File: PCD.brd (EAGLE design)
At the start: 64 x 56 mm, 15 parts, among them J1 M40-SOCKET-BELOW, J2 DC IN, J4 DC IN, J5 OLED, J7 M14PTH, J8 M06-PLAIN, J9 M06-PLAIN

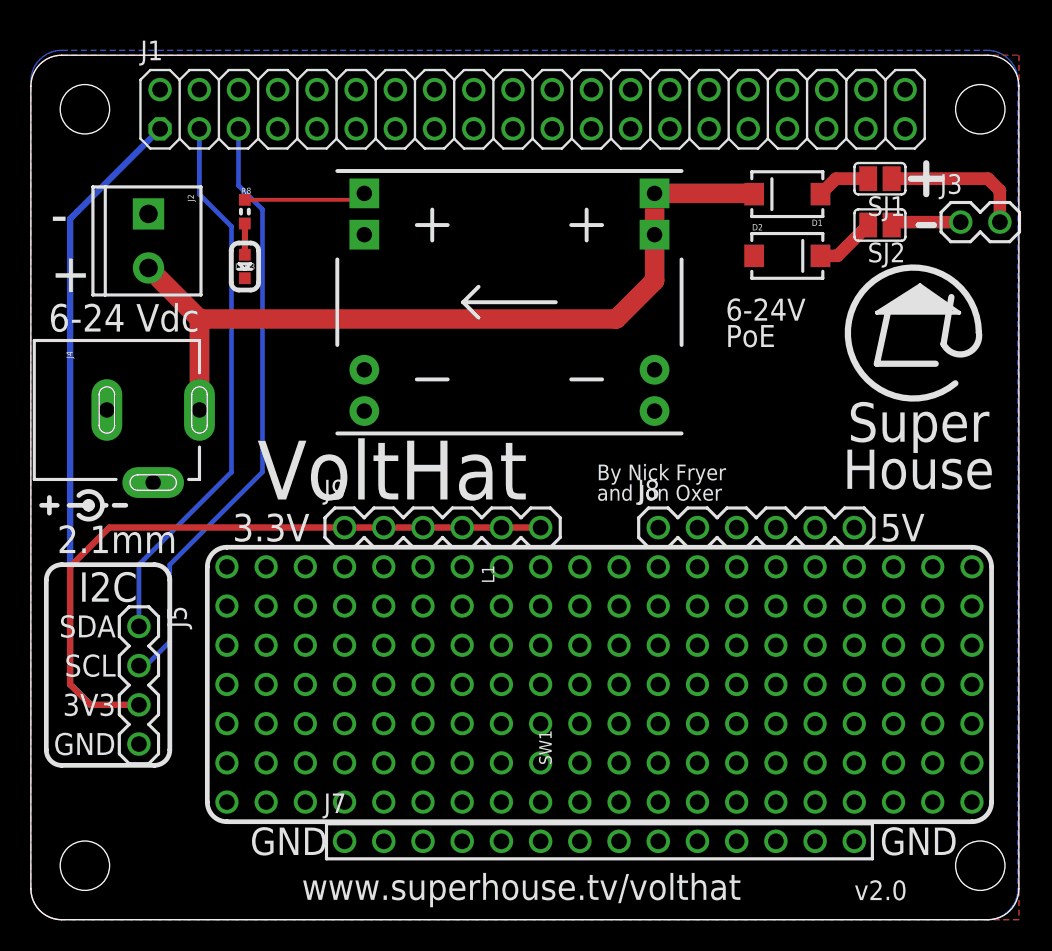
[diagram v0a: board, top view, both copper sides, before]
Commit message: Basic schematic and routing. Time to ponder it for a while.
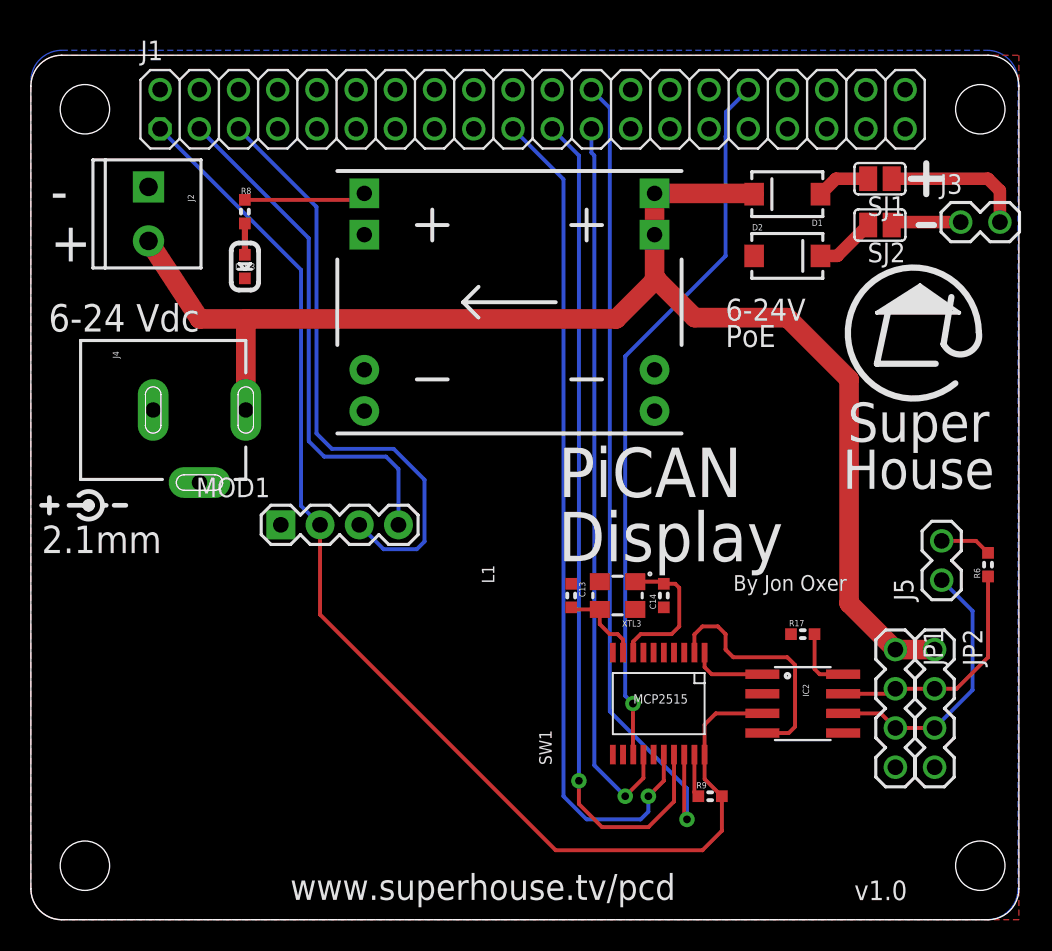
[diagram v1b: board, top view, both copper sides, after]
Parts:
- removed J7: M14PTH, freetronics-jon:1X14
- removed J8, J9: M06-PLAIN, SuperHouse-Connectors:1X06
- added C13, C14: 15pF, SuperHouse-DiscreteSemi:C0603
- added IC2: TCAN332DR, SuperHouse-ICs:SO08
- added IC4: MCP2515, SuperHouse-ICs:TSSOP20
- added JP1, JP2: CAN, SuperHouse-Connectors:1X04-P
- added MOD1: OLED-I2C128X64-0.96, SuperHouse-Displays:OLED-128X64-0.96
- added R17, R9: 10K, SuperHouse-DiscreteSemi:R0603
- added R6: 120R, SuperHouse-DiscreteSemi:R0603
- added XTL3: 16MHz, SuperHouse-Oscillators:CRYSTAL-SMD-3X2
- J5: value OLED -> CAN Termination; device SuperHouse-Connectors:1X04 -> SuperHouse-Connectors:1X02-P
- moved J5 52.1 mm to (59.0, 22.0), turned to 90 degrees
- moved J4 3.00 mm to (0.22, 33.0)
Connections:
- new net CANH: IC2.7, JP1.2, JP2.2, R6.1
- new net CANL: IC2.6, J5.1, JP1.3, JP2.3
- new net IO12: IC4.13, J1.32
- new net IO8: IC4.18, J1.24
- new net MISO: IC4.17, J1.21
- new net MOSI: IC4.16, J1.19
- new net N$26: IC2.8, R17.2
- new net N$28: IC2.1, IC4.1
- new net N$29: IC2.4, IC4.2
- new net N$3: J5.2, R6.2
- new net N$30: C13.2, IC4.9, XTL3.3
- new net N$48: C14.2, IC4.8, XTL3.1
- new net N$49: IC4.19, R9.1
- new net SCK: IC4.14, J1.23
- net 3.3V: now also IC2.3, IC4.20, MOD1.VCC, R9.2; no longer J5.3, J9.1, J9.2, J9.3, J9.4, J9.5, J9.6
- net 5V: no longer J8.1, J8.2, J8.3, J8.4, J8.5, J8.6
- net GND: now also C13.1, C14.1, IC2.2, IC4.10, JP1.4, JP2.4, MOD1.GND, R17.1, XTL3.2, XTL3.4; no longer J5.4, J7.1, J7.10, J7.11, J7.12, J7.13, J7.14, J7.2, J7.3, J7.4, J7.5, J7.6, J7.7, J7.8, J7.9
- net POS: now also JP1.1, JP2.1
- net SCL: now also MOD1.SCL; no longer J5.2
- net SDA: now also MOD1.SDA; no longer J5.1
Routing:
- net MOSI: track 0.00 -> 55.0 mm, vias 0 -> 1
- net MISO: track 0.00 -> 55.0 mm, vias 0 -> 1
- net IO8: track 0.00 -> 54.1 mm, vias 0 -> 1
- net SCK: track 0.00 -> 47.3 mm, vias 0 -> 1
- net IO12: track 0.00 -> 46.6 mm, vias 0 -> 1
- net POS: track 53.3 -> 91.2 mm
- net CANL: track 0.00 -> 17.7 mm
- net N$29: track 0.00 -> 15.8 mm
- net CANH: track 0.00 -> 15.6 mm
- net N$48: track 0.00 -> 9.62 mm
- net 3.3V: track 87.6 -> 80.0 mm
- net N$30: track 0.00 -> 5.62 mm
- net N$28: track 0.00 -> 4.87 mm
- net N$26: track 0.00 -> 4.25 mm
- net N$3: track 0.00 -> 3.32 mm, vias 1 -> 0
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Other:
- board text added: "By Jon Oxer"
- board text added: "PiCAN Display"
- board text added: "v1.0"
- board text added: "www.superhouse.tv/pcd"
- board text removed: "3.3V"
- board text removed: "3V3"
- board text removed: "5V"
- board text removed: "By Nick Fryer and Jon Oxer"
- board text removed: "GND"
- board text removed: "I2C"
- board text removed: "SCL"
- board text removed: "SDA"
- board text removed: "VoltHat"
- board text removed: "v2.0"
- board text removed: "www.superhouse.tv/volthat"
